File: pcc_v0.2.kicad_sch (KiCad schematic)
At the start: 66 parts, among them J2 Conn_01x04_Socket, J3 Conn_01x02_Socket, J4 Conn_02x14_Counter_Clockwise, J6 Conn_01x04_Socket, J7 Conn_01x04_Socket, J8 Conn_01x02_Socket, K3 PCN-112D3MHZ_000, K4 Relay_SPDT, U10 LM2904B, U2 4N35, U3 4N35, U5 DMN63D8L-7, U7 Teensy4.0, U8 SN65HVD230, U9 LM1117T-5.0

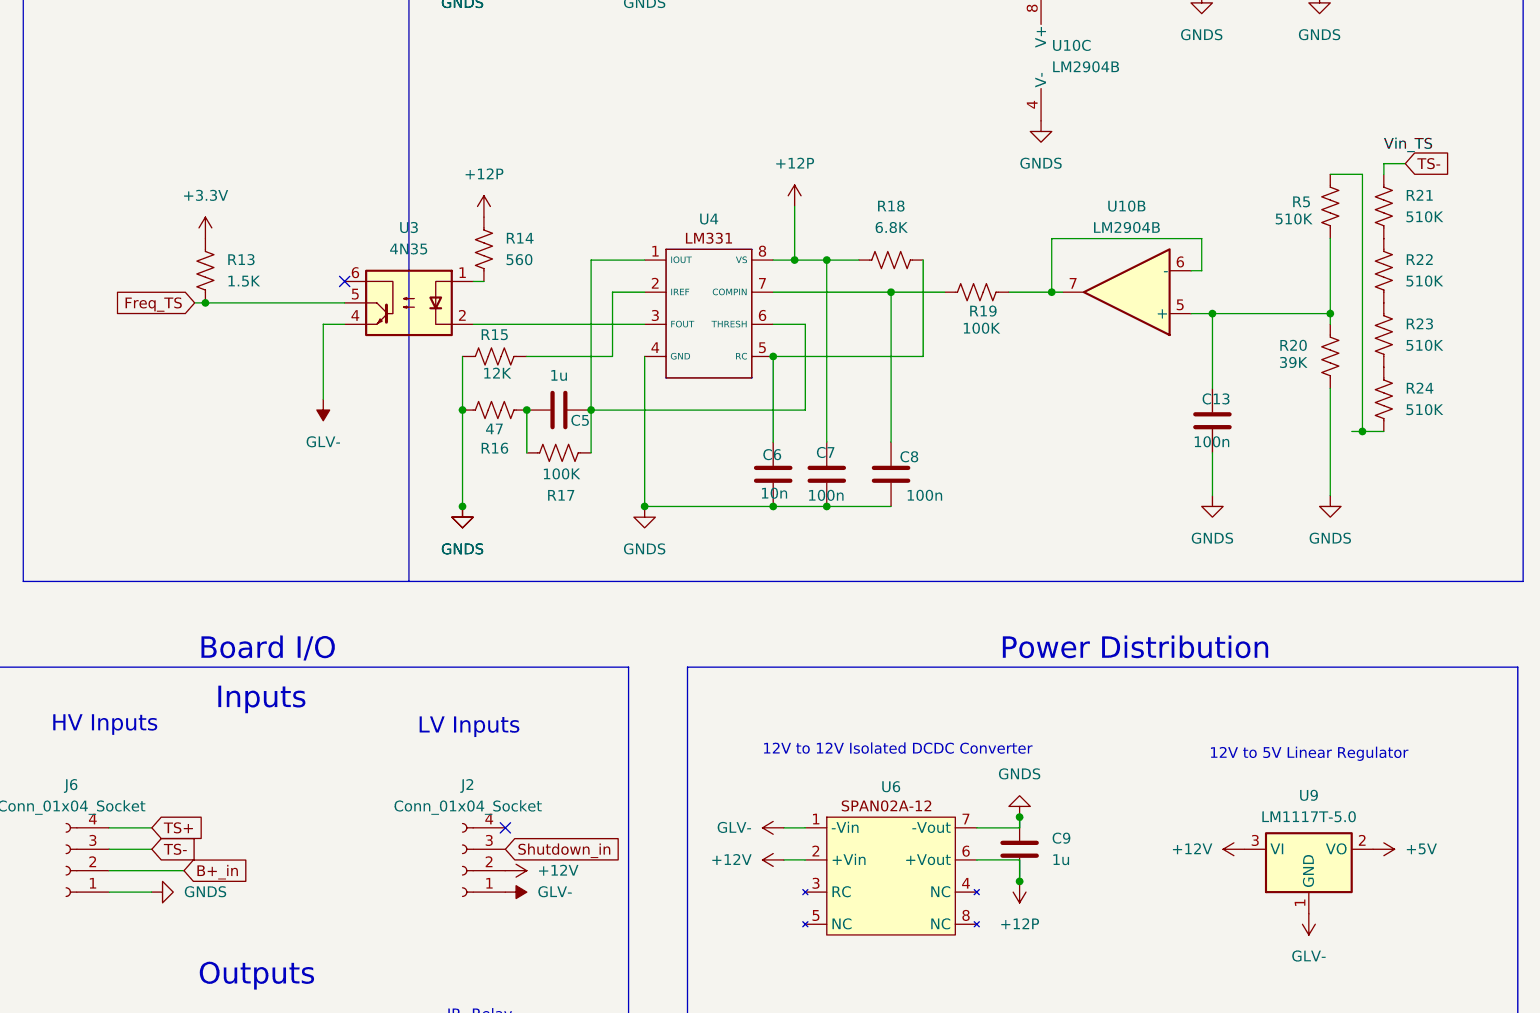
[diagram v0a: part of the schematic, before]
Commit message: Add files via upload
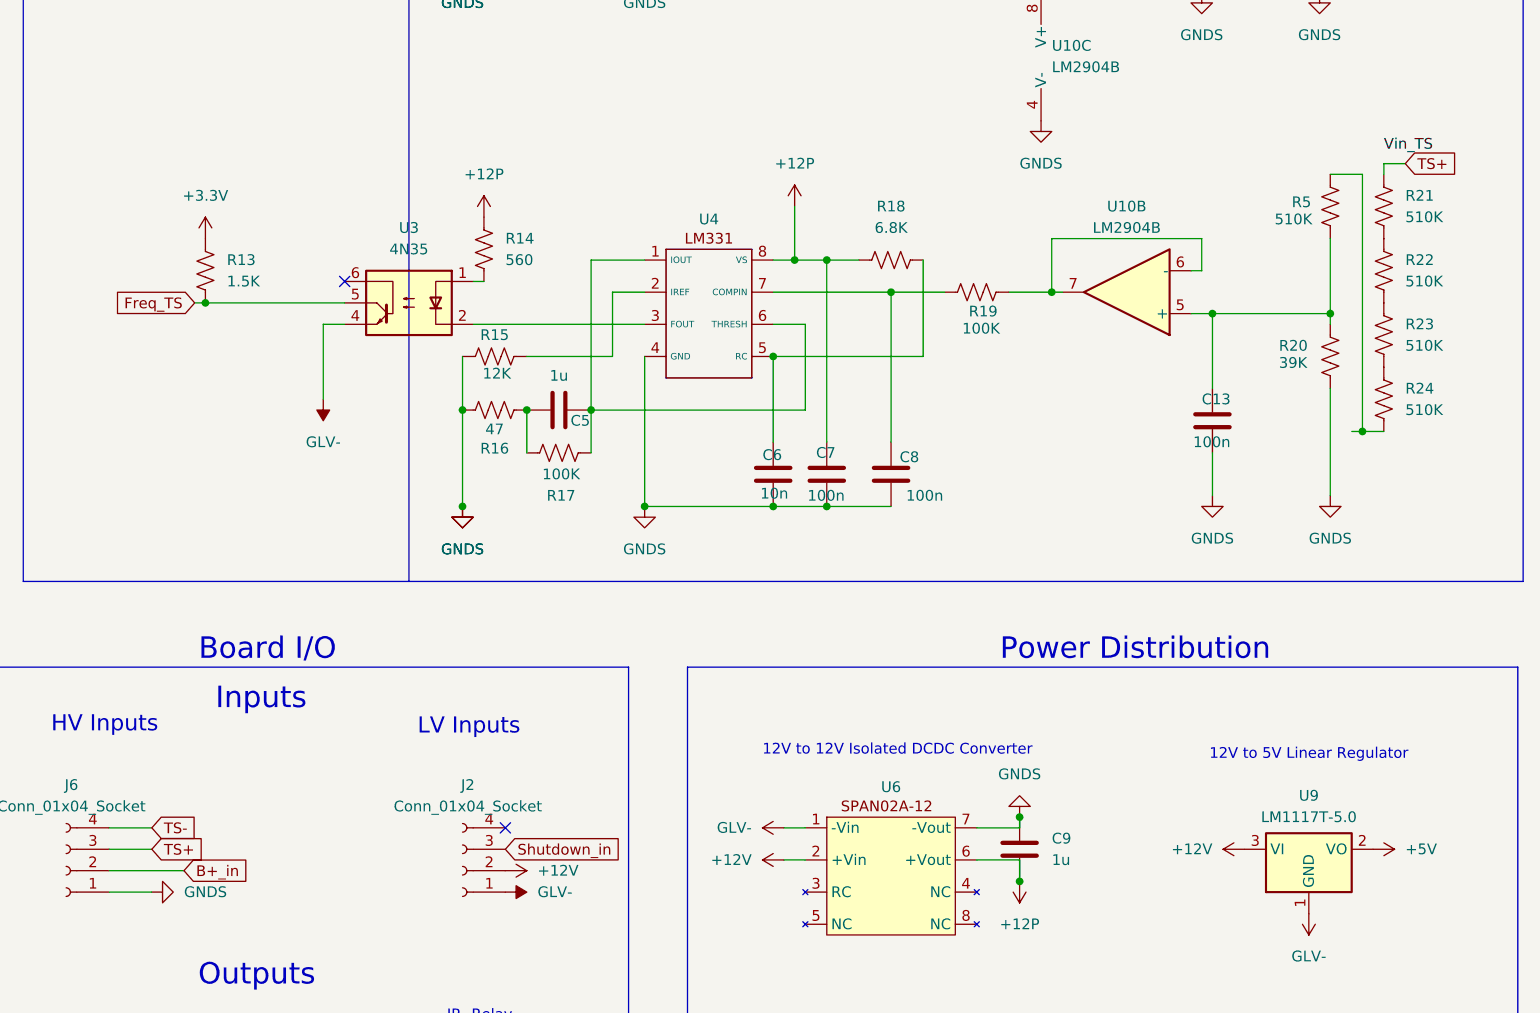
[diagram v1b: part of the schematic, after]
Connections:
- net TS+: now also J6.3 (Pin_3), R21.1; no longer J6.4 (Pin_4)
- net TS-: now also J6.4 (Pin_4); no longer J6.3 (Pin_3), R21.1
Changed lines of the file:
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@@
 		)
 	)
-	(global_label "TS-"
+	(global_label "TS+"
 		(shape input)
 		(at 377.19 100.33 0)
@@
 		)
 	)
-	(global_label "TS+"
+	(global_label "TS-"
 		(shape input)
 		(at 228.6 179.07 0)
@@
 		)
 	)
-	(global_label "TS-"
+	(global_label "TS+"
 		(shape input)
 		(at 228.6 181.61 0)

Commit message: Add files via upload
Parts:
- added C14, C15, C16, C17: 100n, Capacitor_SMD:C_0805_2012Metric, symbol Device:C
- added D3: RF01VM2S, Diode_SMD:D_SOD-323, symbol Diode:RF01VM2S
- added D4: ESD562-Q1, Package_TO_SOT_SMD:SOT-23-3, symbol Power_Protection:ESDA5V3L
- added F1, F2: Fuse, Fuse:Fuse_1206_3216Metric, symbol Device:Fuse
- added J5: Conn_01x02_Socket, Connector_Molex:Molex_Mini-Fit_Jr_5566-02A2_2x01_P4.20mm_Vertical, symbol Connector:Conn_01x02_Socket
- added K5: PCN-112D3MHZ_000, PCN_112D3HMZ:RELAY_PCN-105D3MHZ_000_TEC, symbol PCN_112D3HMZ:PCN-112D3MHZ_000
- added Q1, Q2: MMBT3906, Package_TO_SOT_SMD:SOT-23, symbol Transistor_BJT:MMBT3906
- added R34, R48: 500k, Resistor_SMD:R_0805_2012Metric, symbol Device:R_US
- added R35, R37, R38, R39, R45, R47, R50, R51: 10k, Resistor_SMD:R_0805_2012Metric, symbol Device:R_US
- added R36, R44: 12k, Resistor_SMD:R_0805_2012Metric, symbol Device:R_US
- added R40, R53, R56: 6k8, Resistor_SMD:R_0805_2012Metric, symbol Device:R_US
- added R41, R49: 2k2, Resistor_SMD:R_0805_2012Metric, symbol Device:R_US
- added R42, R52, R55: 20k, Resistor_SMD:R_0805_2012Metric, symbol Device:R_US
- added R43, R46: R, Resistor_THT:R_Axial_DIN0207_L6.3mm_D2.5mm_P7.62mm_Horizontal, symbol Device:R
- added R54, R57, R58, R59, R60, R61: 5k, Resistor_SMD:R_2512_6332Metric, symbol Device:R_US
- added U11: LM393, Package_SO:SOIC-8_3.9x4.9mm_P1.27mm, symbol Comparator:LM393
- added U12, U14: 4N35, Package_DIP:DIP-6_W7.62mm_Socket, symbol Isolator:4N35
- added U13, U15: DMN63D8L-7, nmos:SOIC_63D8L-7_DIO, symbol 2025-01-28_19-23-41:DMN63D8L-7
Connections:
- net +12P: now also C14.1, C16.1, R36.1, R43.1, R44.1, R46.1, U11.8 (V+), U12.2, U14.2
- net +12V: now also D3.1 (K), K5.1, Q1.3 (C), Q2.3 (C), R38.2, R50.2
- net CANH: now also D4.1 (K)
- net CANL: now also D4.2 (K)
- net GLV-: now also D4.3 (A), K5.4, R39.2, R40.2, R51.2, R53.2, R56.2, U12.6, U13.2 (D), U14.6, U15.3 (S); no longer D1.2 (A), J8.1 (Pin_1), K4.A2
- net GNDS: now also C15.2, C17.2, R35.2, R37.2, R45.2, R47.2, U11.4 (V-)
- net Shutdown_in: now also R55.1
- net TS+: now also R54.1
- net TS-: now also R59.1
- net Pre_Dis: now reaches U7.12 (10_CS_MQSR)
- net Pre_Dis: now also J4.12 (Pin_12), U15.1 (G)
- net IR-: now reaches U7.14 (12_MISO_MQSL)
- net IR-: now also J4.14 (Pin_14), U13.1 (G)
- net at U7.4 (2_OUT2): now also R55.2, R56.1
- net at U7.7 (5_IN2): now also R40.1, R42.2
- net at U7.8 (6_OUT1D): now also R52.2, R53.1
- new net: D3.2 (A), K5.2, U13.3 (S)
- new net: Q1.1 (B), R38.1, U12.5
- new net: D1.2 (A), K4.A2, U15.2 (D)
- new net: F2.1, R58.2
- new net: C15.1, R34.1, R36.2, R37.1, U11.3 (+)
- new net: R34.2, R41.1, U11.1
- new net: C14.2, R35.1, R43.2, U11.2 (-)
- new net: C17.1, R44.2, R45.1, R48.1, U11.5 (+)
- new net: R48.2, R49.1, U11.7
- new net: F1.1, R61.2
- new net: R54.2, R57.1
- new net: R57.2, R58.1
- new net: Q2.1 (B), R50.1, U14.5
- new net: R59.2, R60.1
- new net: R60.2, R61.1
- new net: C16.2, R46.2, R47.1, U11.6 (-)
- new net: R49.2, U14.1
- new net: R41.2, U12.1
- new net IR-_GND: J8.1 (Pin_1), K5.3
- new net PDOC_OK1: Q1.2 (E), R39.1, R42.1
- new net PDOC_OK2: Q2.2 (E), R51.1, R52.1
- new net TSMP+: F2.2, J5.2 (Pin_2)
- new net TSMP-: F1.2, J5.1 (Pin_1)
- no-connect marks 67 -> 62
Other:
- note added: "IR- Precharge Control"
- note added: "TSMP"
- moved on the sheet: C1, C10, C11, C12, C13, C2, C3, C4, C5, C6, C7, C8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

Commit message: Add files via upload
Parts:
- removed C16, C17: 100n, Capacitor_SMD:C_0805_2012Metric, symbol Device:C
- removed D2, D3: RF01VM2S, Diode_SMD:D_SOD-323, symbol Diode:RF01VM2S
- removed F1: Fuse, Fuse:Fuse_1206_3216Metric, symbol Device:Fuse
- removed J5: Conn_01x02_Socket, Connector_Molex:Molex_Mini-Fit_Jr_5566-02A2_2x01_P4.20mm_Vertical, symbol Connector:Conn_01x02_Socket
- removed K3, K5: PCN-112D3MHZ_000, PCN_112D3HMZ:RELAY_PCN-105D3MHZ_000_TEC, symbol PCN_112D3HMZ:PCN-112D3MHZ_000
- removed Q1, Q2: MMBT3906, Package_TO_SOT_SMD:SOT-23, symbol Transistor_BJT:MMBT3906
- removed R34, R48: 500k, Resistor_SMD:R_0805_2012Metric, symbol Device:R_US
- removed R35, R37, R38, R39, R45, R47, R50, R51: 10k, Resistor_SMD:R_0805_2012Metric, symbol Device:R_US
- removed R36, R44: 12k, Resistor_SMD:R_0805_2012Metric, symbol Device:R_US
- removed R41, R49: 2k2, Resistor_SMD:R_0805_2012Metric, symbol Device:R_US
- removed R42, R52: 20k, Resistor_SMD:R_0805_2012Metric, symbol Device:R_US
- removed R46: R, Resistor_THT:R_Axial_DIN0207_L6.3mm_D2.5mm_P7.62mm_Horizontal, symbol Device:R
- removed R54, R57, R58, R59, R60, R61: 5k, Resistor_SMD:R_2512_6332Metric, symbol Device:R_US
- removed U11: LM393, Package_SO:SOIC-8_3.9x4.9mm_P1.27mm, symbol Comparator:LM393
- removed U12, U14: 4N35, Package_DIP:DIP-6_W7.62mm_Socket, symbol Isolator:4N35
- removed U13, U5: DMN63D8L-7, nmos:SOIC_63D8L-7_DIO, symbol 2025-01-28_19-23-41:DMN63D8L-7
- added D5, D6: RF01VM2S, Diode_SMD:D_SOD-323, symbol Diode:RF01VM2S
- added F3: Fuse, Fuse:Fuse_1206_3216Metric, symbol Device:Fuse
- added J9: Conn_01x04_Socket, Connector_Molex:Molex_Mini-Fit_Jr_5566-04A2_2x02_P4.20mm_Vertical, symbol Connector:Conn_01x04_Socket
- added Q1, Q2: IRLZ44N, Package_TO_SOT_THT:TO-220-3_Vertical, symbol Transistor_FET:IRLZ44N
- added R44: R, Connector_PinSocket_2.00mm:PinSocket_1x02_P2.00mm_Vertical, symbol Device:R
- added R62, R63, R64, R65, R68, R69, R70, R71, R72, R73: 3k, Resistor_SMD:R_2512_6332Metric, symbol Device:R_US
- added R66, R67: 4k, Resistor_SMD:R_0805_2012Metric, symbol Device:R_US
- R43: footprint Resistor_THT:R_Axial_DIN0207_L6.3mm_D2.5mm_P7.62mm_Horizontal -> Connector_PinSocket_2.00mm:PinSocket_1x02_P2.00mm_Vertical
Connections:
- net +12P: no longer C14.1, R43.1
- net +3.3V: now also R43.1, R44.1
- net GLV-: now also C14.2, C15.2, Q1.3 (S), Q2.3 (S)
- net GNDS: no longer C15.2
- net IR+: now also Q2.1 (G)
- net IR+_GND: now also D6.2 (A), Q2.2 (D)
- net IR-_GND: now also D5.2 (A), Q1.2 (D)
- net Shutdown_in: now also D5.1 (K), D6.1 (K)
- net TS+: now also R62.1, R66.2
- net TS-: now also R63.1, R67.2
- net TSMP+: now also J9.4 (Pin_4), R72.2; no longer F2.2
- net TSMP-: now also J9.3 (Pin_3), R73.2
- net at F2.1: now also R66.1
- net at C15.1: now also R53.1, U7.8 (6_OUT1D), R44.2
- net at R43.2: now also C14.1, R40.1, U7.7 (5_IN2); no longer C14.2
- net IR- renamed PreDis_IR-
- net PreDis_IR-: now also U15.1 (G), Q1.1 (G)
- removed net Pre_Dis: J4.12 (Pin_12), U15.1 (G), U7.12 (10_CS_MQSR)
- new net: F3.1, R67.1
- new net: R70.2, R72.1
- new net: R62.2, R64.1
- new net: R71.2, R73.1
- new net: R69.2, R71.1
- new net: R64.2, R68.1
- new net: R63.2, R65.1
- new net: R65.2, R69.1
- new net: R68.2, R70.1
- new net TSMP+_Fused: F2.2, J9.2 (Pin_2)
- new net TSMP-_Fused: F3.2, J9.1 (Pin_1)
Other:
- moved on the sheet: F2, R43
